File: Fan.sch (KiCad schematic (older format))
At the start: 12 parts, among them Q2 MOSFET_N, Q3 NMOS, Q4 NMOS, U4 OPA4170, U6 MCP4801

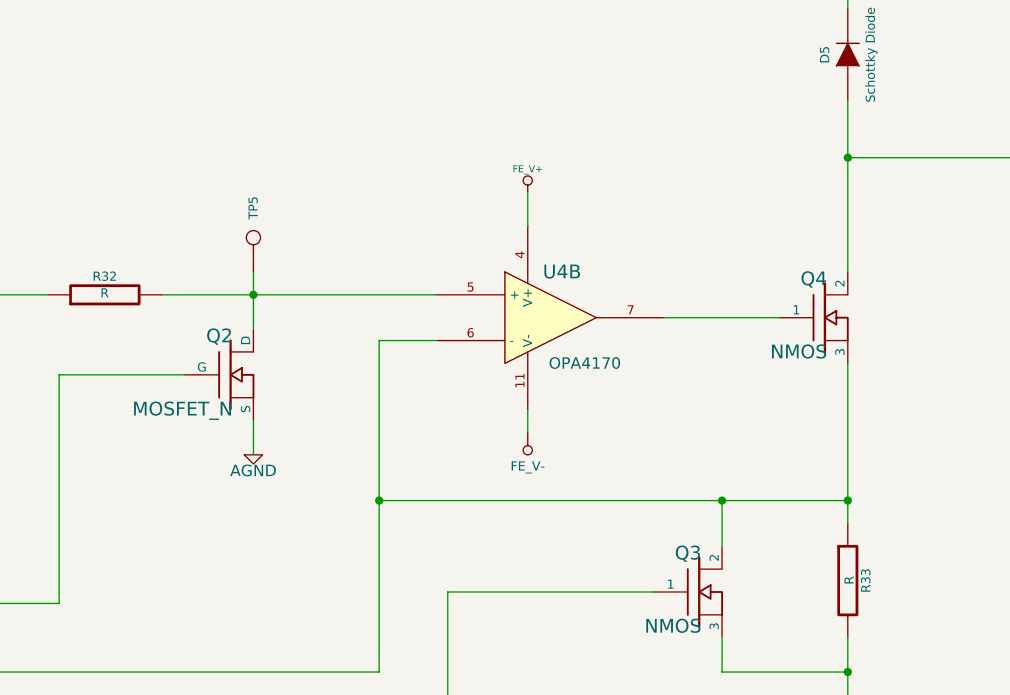
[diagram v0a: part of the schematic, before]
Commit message: Layout v17.0
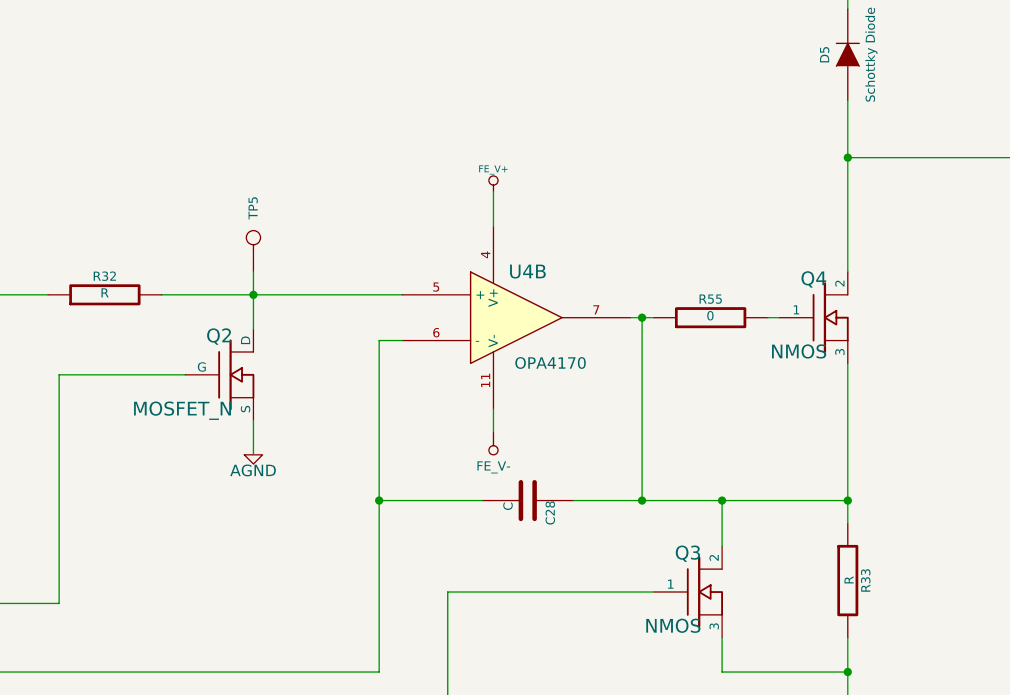
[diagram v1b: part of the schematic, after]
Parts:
- added C28: C, ~, symbol C
- added R55: 0, ~, symbol R
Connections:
- net CURR_MEAS: now also C28.2; no longer Q3.2, Q4.3, R33.1
- net at U4.7: now also Q3.2, Q4.3, R33.1, C28.1, R55.1; no longer Q4.1
- new net: Q4.1, R55.2
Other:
- moved on the sheet: U4B
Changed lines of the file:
@@
 Sheet 6 9
 Title ""
-Date "22 mar 2014"
+Date "23 mar 2014"
 Rev ""
 Comp ""
@@
 L LM324 U4
 U 2 1 52F5F7EF
-P 6350 2750
-F 0 "U4" H 6400 2950 60  0000 C CNN
-F 1 "OPA4170" H 6500 2550 50  0000 C CNN
-F 2 "~" H 6350 2750 60  0000 C CNN
-F 3 "~" H 6350 2750 60  0000 C CNN
-	2    6350 2750
-	1    0    0    -1
-$EndComp
-Wire Wire Line
-	6850 2750 7350 2750
+P 6200 2750
+F 0 "U4" H 6250 2950 60  0000 C CNN
+F 1 "OPA4170" H 6350 2550 50  0000 C CNN
+F 2 "~" H 6200 2750 60  0000 C CNN
+F 3 "~" H 6200 2750 60  0000 C CNN
+	2    6200 2750
+	1    0    0    -1
+$EndComp
 Wire Wire Line
 	7650 2950 7650 3650
@@
 	7650 4150 7650 4400
 Wire Wire Line
-	5850 2850 5600 2850
+	5700 2850 5600 2850
 Wire Wire Line
 	5600 2850 5600 4300
 Wire Wire Line
-	6250 3150 6250 3250
-Wire Wire Line
-	6250 2200 6250 2350
+	6100 3150 6100 3250
+Wire Wire Line
+	6100 2200 6100 2350
 Wire Wire Line
 	5050 3200 5050 3350
@@
 Connection ~ 7650 4300
 Wire Wire Line
-	4650 2650 5850 2650
+	4650 2650 5700 2650
 $Comp
 L MOSFET_N Q2
@@
 FAN_MODE
 Wire Wire Line
-	5600 3550 7650 3550
-Wire Wire Line
 	7100 3750 7100 3550
 Connection ~ 7100 3550
@@
 	5900 4750 2500 4750
 $Comp
-L +12C #PWR045
+L +12C #PWR57
 U 1 1 52F9D6B5
 P 7650 650
-F 0 "#PWR045" H 7650 620 30  0001 C CNN
+F 0 "#PWR57" H 7650 620 30  0001 C CNN
 F 1 "+12C" H 7650 760 40  0000 C CNN
 F 2 "" H 7650 650 60  0000 C CNN
@@
 	1700 3000 2200 3000
 $Comp
-L +5V #PWR046
+L +5V #PWR52
 U 1 1 530B6076
 P 3000 1700
-F 0 "#PWR046" H 3000 1790 20  0001 C CNN
+F 0 "#PWR52" H 3000 1790 20  0001 C CNN
 F 1 "+5V" H 3000 1790 30  0000 C CNN
 F 2 "" H 3000 1700 60  0000 C CNN
@@
 L FE_V- #PWR56
 U 1 1 5312A372
-P 6250 3250
-F 0 "#PWR56" H 6250 3450 40  0001 C CNN
-F 1 "FE_V-" H 6250 3400 40  0000 C CNN
-F 2 "" H 6250 3250 60  0000 C CNN
-F 3 "" H 6250 3250 60  0000 C CNN
-	1    6250 3250
+P 6100 3250
+F 0 "#PWR56" H 6100 3450 40  0001 C CNN
+F 1 "FE_V-" H 6100 3400 40  0000 C CNN
+F 2 "" H 6100 3250 60  0000 C CNN
+F 3 "" H 6100 3250 60  0000 C CNN
+	1    6100 3250
 	-1   0    0    1
 $EndComp
 $Comp
-L FE_V+ #PWR047
+L FE_V+ #PWR55
 U 1 1 5312A378
-P 6250 2200
-F 0 "#PWR047" H 6250 2300 30  0001 C CNN
-F 1 "FE_V+" H 6250 2300 30  0000 C CNN
-F 2 "" H 6250 2200 60  0000 C CNN
-F 3 "" H 6250 2200 60  0000 C CNN
-	1    6250 2200
-	1    0    0    -1
-$EndComp
-$Comp
-L AGND #PWR048
+P 6100 2200
+F 0 "#PWR55" H 6100 2300 30  0001 C CNN
+F 1 "FE_V+" H 6100 2300 30  0000 C CNN
+F 2 "" H 6100 2200 60  0000 C CNN
+F 3 "" H 6100 2200 60  0000 C CNN
+	1    6100 2200
+	1    0    0    -1
+$EndComp
+$Comp
+L AGND #PWR59
 U 1 1 53198B9B
 P 8350 800
-F 0 "#PWR048" H 8350 800 40  0001 C CNN
+F 0 "#PWR59" H 8350 800 40  0001 C CNN
 F 1 "AGND" H 8350 730 50  0000 C CNN
 F 2 "" H 8350 800 60  0000 C CNN
@@
 $EndComp
 $Comp
-L AGND #PWR049
+L AGND #PWR58
 U 1 1 53198BAA
 P 7650 4400
-F 0 "#PWR049" H 7650 4400 40  0001 C CNN
+F 0 "#PWR58" H 7650 4400 40  0001 C CNN
 F 1 "AGND" H 7650 4330 50  0000 C CNN
 F 2 "" H 7650 4400 60  0000 C CNN
@@
 $EndComp
 $Comp
-L AGND #PWR050
+L AGND #PWR54
 U 1 1 53198BB9
 P 5050 3350
-F 0 "#PWR050" H 5050 3350 40  0001 C CNN
+F 0 "#PWR54" H 5050 3350 40  0001 C CNN
 F 1 "AGND" H 5050 3280 50  0000 C CNN
 F 2 "" H 5050 3350 60  0000 C CNN
@@
 $EndComp
 $Comp
-L AGND #PWR051
+L AGND #PWR53
 U 1 1 53198BC8
 P 3000 3600
-F 0 "#PWR051" H 3000 3600 40  0001 C CNN
+F 0 "#PWR53" H 3000 3600 40  0001 C CNN
 F 1 "AGND" H 3000 3530 50  0000 C CNN
 F 2 "" H 3000 3600 60  0000 C CNN
@@
 $EndComp
 $Comp
-L AGND #PWR052
+L AGND #PWR51
 U 1 1 53198BD7
 P 2400 1850
-F 0 "#PWR052" H 2400 1850 40  0001 C CNN
+F 0 "#PWR51" H 2400 1850 40  0001 C CNN
 F 1 "AGND" H 2400 1780 50  0000 C CNN
 F 2 "" H 2400 1850 60  0000 C CNN
@@
 	0    -1   -1   0
 $EndComp
+$Comp
+L R R55
+U 1 1 532EBE1B
+P 7050 2750
+F 0 "R55" V 7130 2750 40  0000 C CNN
+F 1 "0" V 7057 2751 40  0000 C CNN
+F 2 "~" V 6980 2750 30  0000 C CNN
+F 3 "~" H 7050 2750 30  0000 C CNN
+	1    7050 2750
+	0    -1   -1   0
+$EndComp
+Wire Wire Line
+	7300 2750 7350 2750
+Wire Wire Line
+	6800 2750 6700 2750
+Wire Wire Line
+	6450 3550 7650 3550
+$Comp
+L C C28
+U 1 1 532EBEBB
+P 6250 3550
+F 0 "C28" H 6250 3650 40  0000 L CNN
+F 1 "C" H 6256 3465 40  0000 L CNN
+F 2 "~" H 6288 3400 30  0000 C CNN
+F 3 "~" H 6250 3550 60  0000 C CNN
+	1    6250 3550
+	0    1    1    0
+$EndComp
+Wire Wire Line
+	6050 3550 5600 3550
+Wire Wire Line
+	6750 2750 6750 3550
+Connection ~ 6750 3550
+Connection ~ 6750 2750
 $EndSCHEMATC

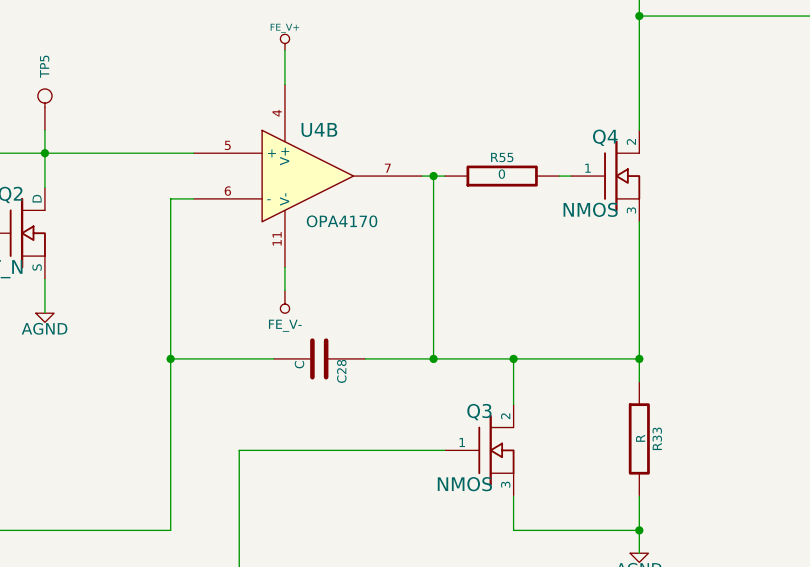
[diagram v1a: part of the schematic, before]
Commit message: Layout v17.1
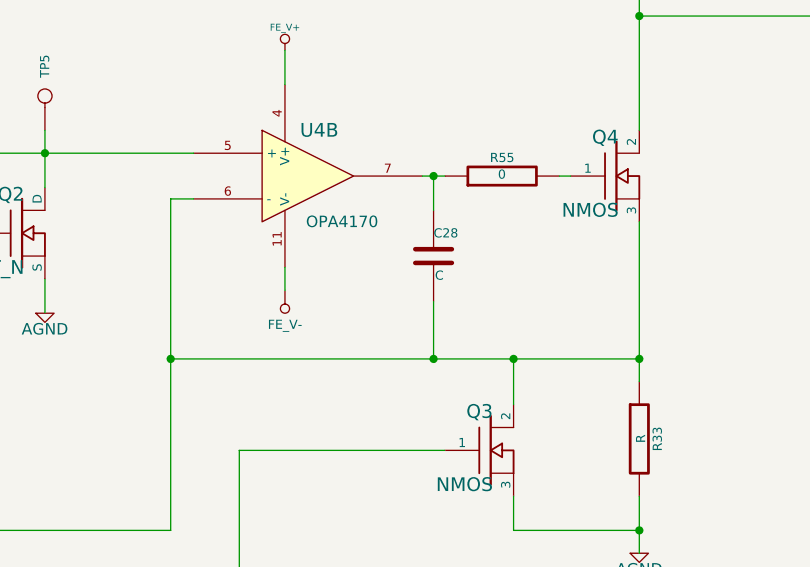
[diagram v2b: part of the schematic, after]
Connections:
- net CURR_MEAS: now also Q3.2, Q4.3, R33.1
- net at C28.1, R55.1, U4.7: no longer Q3.2, Q4.3, R33.1
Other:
- moved on the sheet: C28
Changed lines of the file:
@@
 	6800 2750 6700 2750
 Wire Wire Line
-	6450 3550 7650 3550
+	5600 3550 7650 3550
 $Comp
 L C C28
 U 1 1 532EBEBB
-P 6250 3550
-F 0 "C28" H 6250 3650 40  0000 L CNN
-F 1 "C" H 6256 3465 40  0000 L CNN
-F 2 "~" H 6288 3400 30  0000 C CNN
-F 3 "~" H 6250 3550 60  0000 C CNN
-	1    6250 3550
-	0    1    1    0
+P 6750 3100
+F 0 "C28" H 6750 3200 40  0000 L CNN
+F 1 "C" H 6756 3015 40  0000 L CNN
+F 2 "~" H 6788 2950 30  0000 C CNN
+F 3 "~" H 6750 3100 60  0000 C CNN
+	1    6750 3100
+	1    0    0    -1
 $EndComp
-Wire Wire Line
-	6050 3550 5600 3550
-Wire Wire Line
-	6750 2750 6750 3550
 Connection ~ 6750 3550
 Connection ~ 6750 2750
+Wire Wire Line
+	6750 2750 6750 2900
+Wire Wire Line
+	6750 3300 6750 3550
 $EndSCHEMATC
